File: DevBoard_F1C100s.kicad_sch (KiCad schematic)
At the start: 51 parts, among them J101 USB_C_Receptacle_USB2.0_16P, J102 Conn_01x22, J103 Conn_01x11, J104 SD_Card, J105 UART0, J106 Conn_01x10, J108 Conn_01x05, SW101 SW0, SW102 SW1, SW103 SW2, SW104 SW3, SW105 RESET, U101 AMS1117, U102 AMS1117-3.3, U103 TPS562201DDCT, U104 W25Q16JVSS, U105 F1C100s, Y101 24Mhz

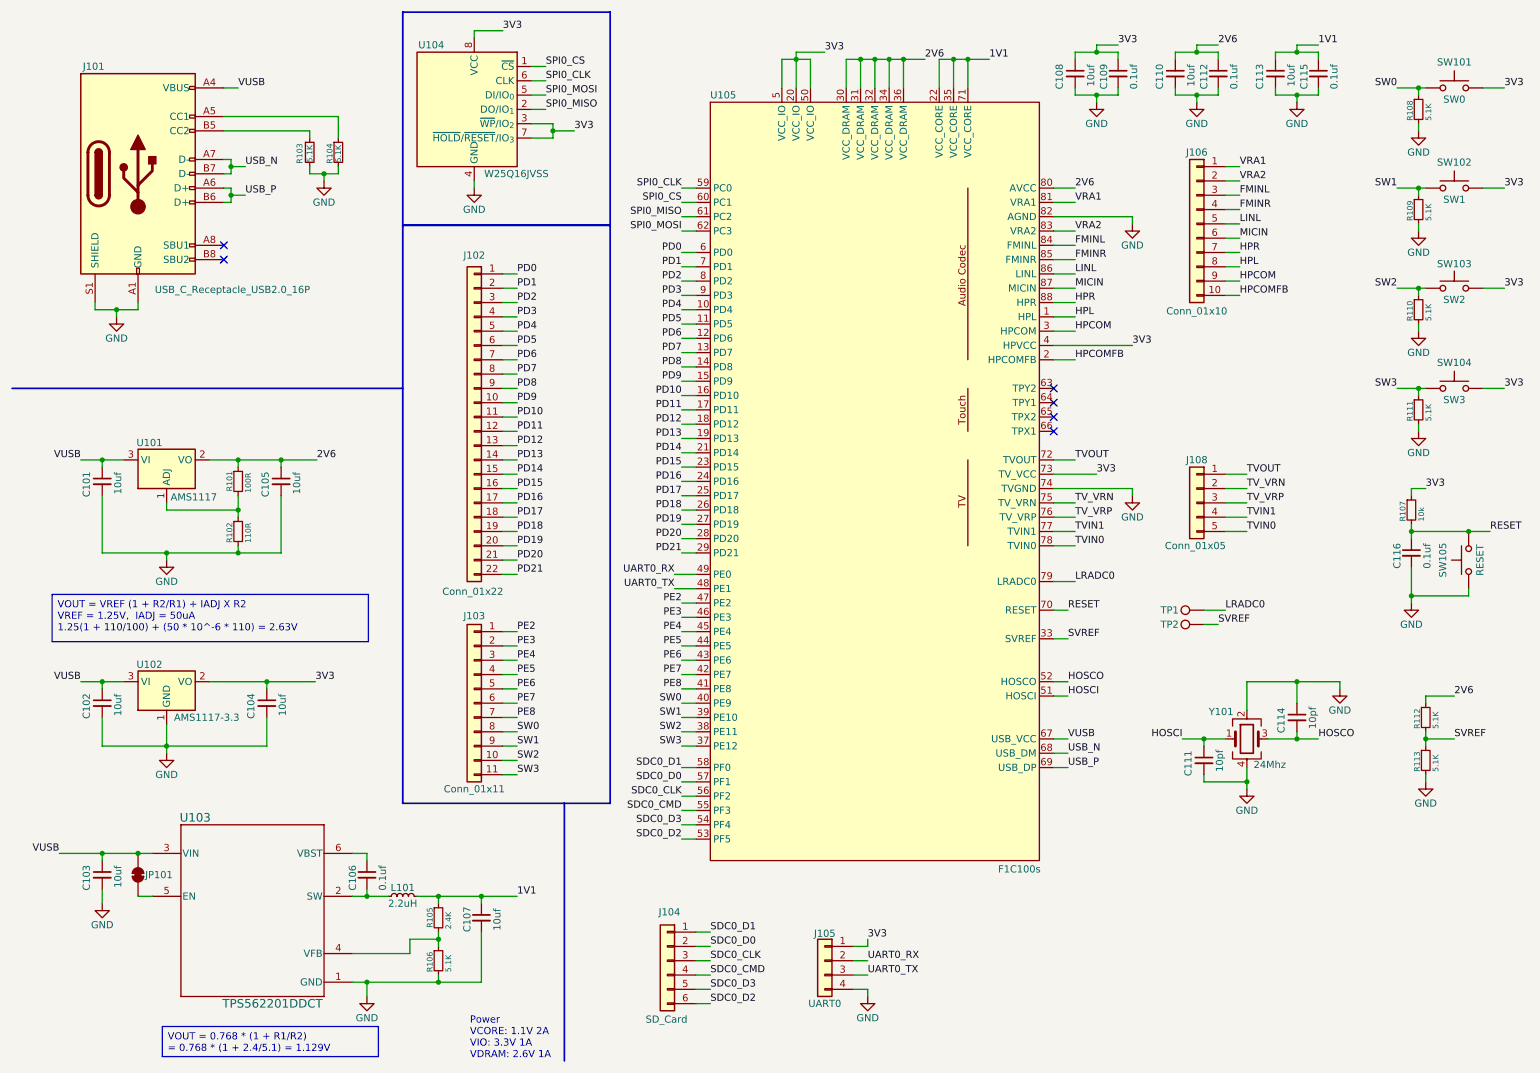
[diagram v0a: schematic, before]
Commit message: Finish design
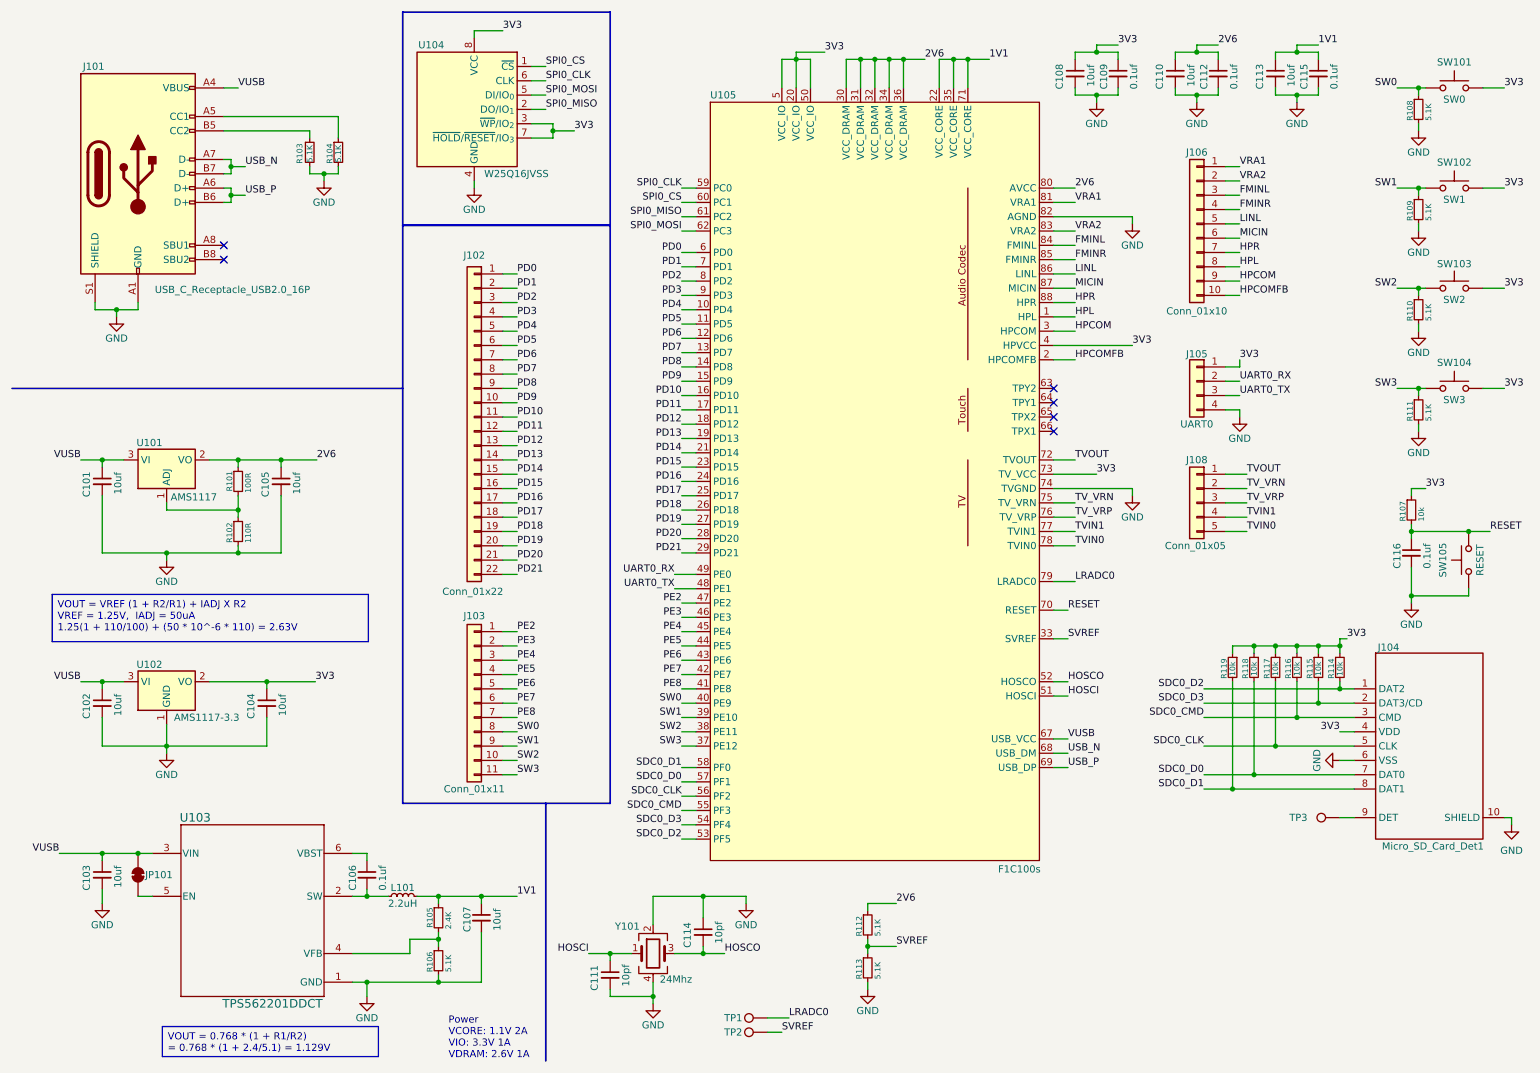
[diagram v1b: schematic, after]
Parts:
- removed J104: SD_Card, Connector_PinHeader_1.00mm:PinHeader_1x06_P1.00mm_Vertical_SMD_Pin1Left, symbol Connector_Generic:Conn_01x06
- added J104: Micro_SD_Card_Det1, sd_card:sd_card_10p, symbol sd_card:Micro_SD_Card_Det1
- added R114, R115, R116, R117, R118, R119: 10k, Resistor_SMD:R_0603_1608Metric_Pad0.98x0.95mm_HandSolder, symbol Device:R_Small
- added TP3: TestPoint, TestPoint:TestPoint_Pad_D1.0mm, symbol Connector:TestPoint
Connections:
- net 3V3: now also J104.4 (VDD), R114.1, R115.1, R116.1, R117.1, R118.1, R119.1
- net GND: now also J104.10 (SHIELD), J104.6 (VSS)
- net SDC0_CLK: now also J104.5 (CLK), R117.2
- net SDC0_CMD: now also J104.3 (CMD), R116.2
- net SDC0_D0: now also J104.7 (DAT0), R118.2
- net SDC0_D1: now also J104.8 (DAT1), R119.2
- net SDC0_D2: now also J104.1 (DAT2), R114.2
- net SDC0_D3: now also J104.2 (DAT3/CD), R115.2
- new net: J104.9 (DET), TP3.1
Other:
- moved on the sheet: C111, C114, J105, R112, R113, TP1, TP2, Y101
